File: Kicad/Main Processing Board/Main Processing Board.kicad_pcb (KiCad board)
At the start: 2 copper layers, 0 parts

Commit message: added 3d models
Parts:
- added 11111: ~, project-library:SDREAD, F.Cu at (118.1, 71.2)
- added 12111: ~, project-library:ARDUCAM_MINI, B.Cu at (101.3, 74.5)
- added AtmosphericSensor1: MS5611-01BA03, MS5611:SON125P500X300X100-8N, F.Cu at (103.8, 75.8)
- added I2CBus1: ~, Connector_JST:JST_SH_BM04B-SRSS-TB_1x04-1MP_P1.00mm_Vertical, F.Cu at (108.9, 54.5)
- added J1: Conn_01x10_MountingPin, Connector_JST:JST_SH_BM10B-SRSS-TB_1x10-1MP_P1.00mm_Vertical, F.Cu at (132.3, 62.4)
- added PowerBoard1: ~, Connector_Molex:Molex_PicoBlade_53047-0410_1x04_P1.25mm_Vertical, F.Cu at (129.9, 77.9)
- added U1: ~, SN74LVC125ANSR:NS14, F.Cu at (121.2, 55.9)
- added U2: Seeed Studio XIAO SAMD21, Seeed Studio XIAO Series Library:XIAO-SAMD21-SMD, B.Cu at (109.5, 56.8)
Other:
- board outline added: 35 x 29.5 mm

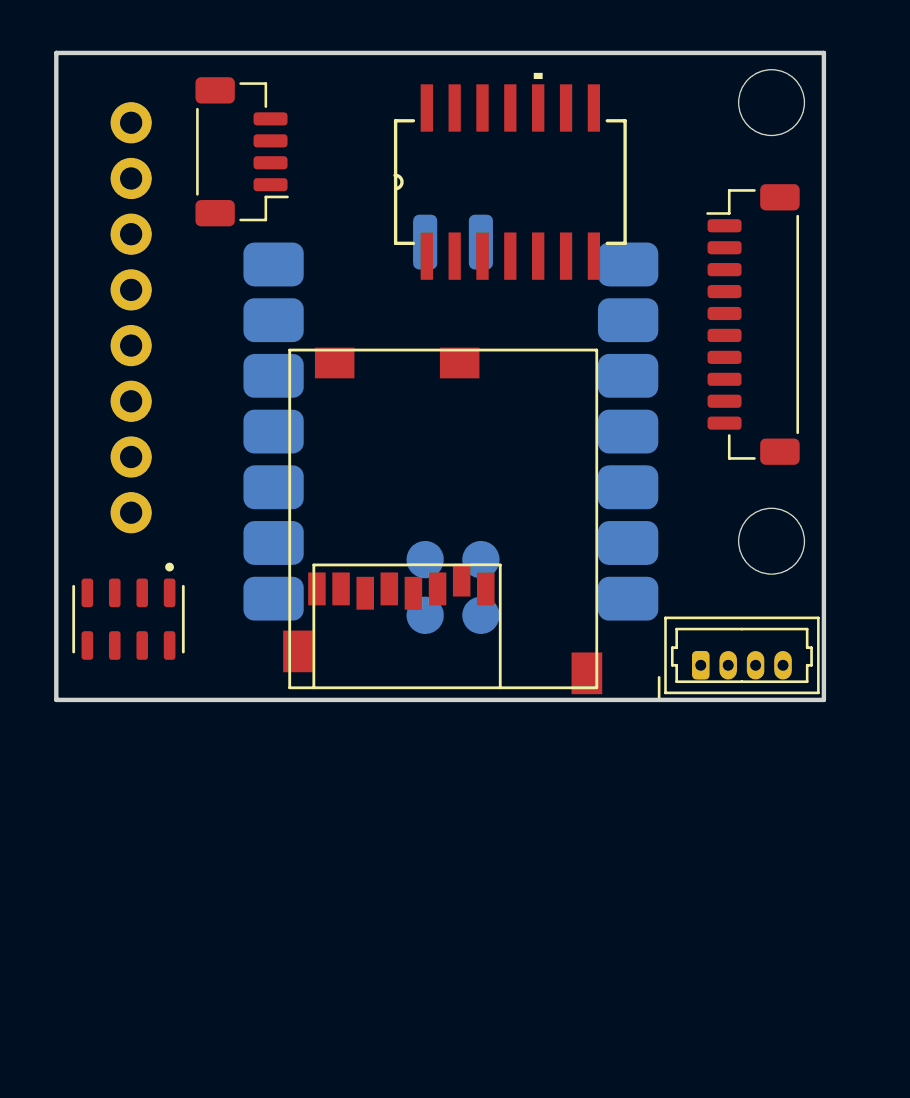
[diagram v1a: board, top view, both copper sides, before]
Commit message: routed pcb
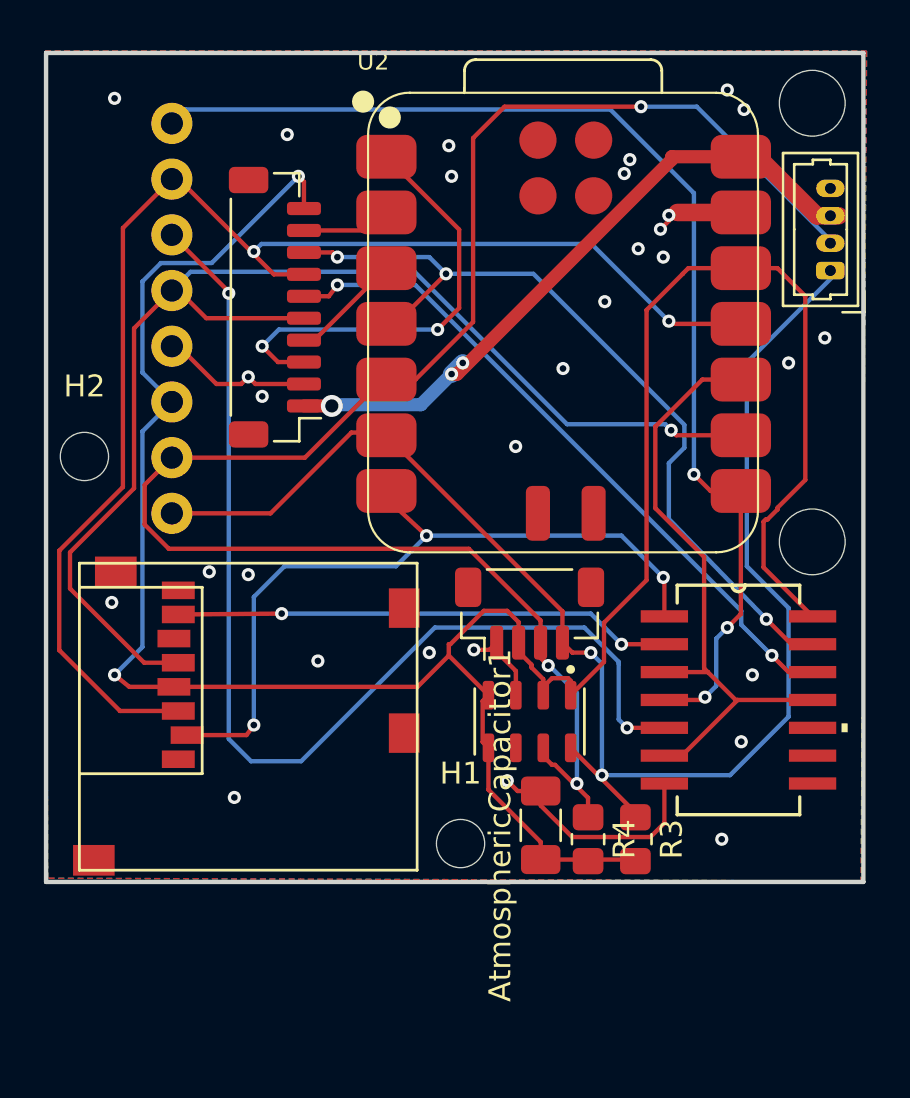
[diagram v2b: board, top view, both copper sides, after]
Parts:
- added AtmosphericCapacitor1: 100nF, Capacitor_SMD:C_1206_3216Metric_Pad1.33x1.80mm_HandSolder, F.Cu at (122.6, 85.2)
- added H1: MountingHole, MountingHole:MountingHole_2.2mm_M2, F.Cu at (118.9, 86.0)
- added H2: MountingHole, MountingHole:MountingHole_2.2mm_M2, F.Cu at (101.8, 68.4)
- added R3: 10K, Resistor_SMD:R_0805_2012Metric_Pad1.20x1.40mm_HandSolder, F.Cu at (126.9, 85.9)
- added R4: 10K, Resistor_SMD:R_0805_2012Metric_Pad1.20x1.40mm_HandSolder, F.Cu at (124.7, 85.9)
- U2: moved to F.Cu
- moved U1 25.8 mm to (131.6, 79.5), turned to 0 degrees
- moved I2CBus1 24.8 mm to (122.0, 75.6), turned to 0 degrees
- moved J1 21.8 mm to (110.4, 61.6), turned to 90 degrees
- moved PowerBoard1 18.9 mm to (135.8, 59.9), turned to 90 degrees
- moved AtmosphericSensor1 18.9 mm to (122.0, 80.5)
- moved U2 16.9 mm to (114.7, 72.9)
- moved 11111 12.7 mm to (109.2, 80.3), turned to -90 degrees
- moved 12111 1.86 mm to (103.2, 74.5)
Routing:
- net +3.3V: track 0.00 -> 117.2 mm, vias 0 -> 2
- net /SDA_I2C: track 0.00 -> 80.0 mm, vias 0 -> 3
- net /SCL_I2C: track 0.00 -> 68.4 mm, vias 0 -> 2
- net /MOSI: track 0.00 -> 61.9 mm, vias 0 -> 2
- net /SCK_SPI: track 0.00 -> 57.8 mm, vias 0 -> 1
- net /CAMERA_CS: track 0.00 -> 52.9 mm, vias 0 -> 3
- net /Camera_MISO: track 0.00 -> 50.3 mm, vias 0 -> 2
- net /Radio_CS: track 0.00 -> 37.8 mm, vias 0 -> 3
- net /SD_CS: track 0.00 -> 34.5 mm, vias 0 -> 3
- net /Radio_MISO: track 0.00 -> 31.1 mm, vias 0 -> 2
- net +5V: track 0.00 -> 31.0 mm, vias 0 -> 3
- net /MISO: track 0.00 -> 28.6 mm
- net GND: track 0.00 -> 25.8 mm, vias 0 -> 30
- net /SD_MISO: track 0.00 -> 22.7 mm, vias 0 -> 2
- net /Radio_EN: track 0.00 -> 20.2 mm, vias 0 -> 2
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- added copper zone on B.Cu, net GND
- added copper zone on F.Cu, net GND
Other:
- board size 35 x 29.5 mm -> 37.3 x 37.8 mm
